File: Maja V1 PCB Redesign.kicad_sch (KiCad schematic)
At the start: 22 parts, among them J1 TYPE-C-31-M-12, J2 AVR-ISP-6, J3 Connector_Generic_Conn_01x04, U1 ATmega32U4-M, U2 PRTR5V0U2X, Y1 Crystal_GND24_Small

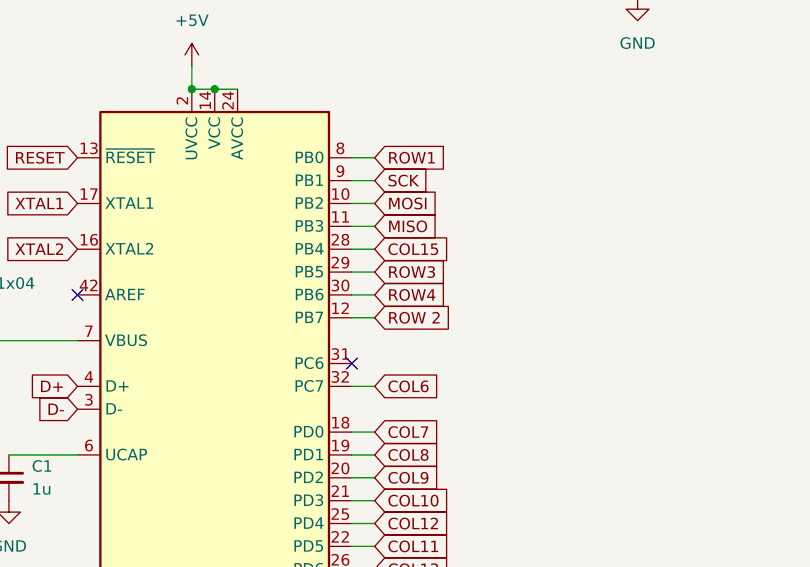
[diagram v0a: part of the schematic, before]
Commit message: routing
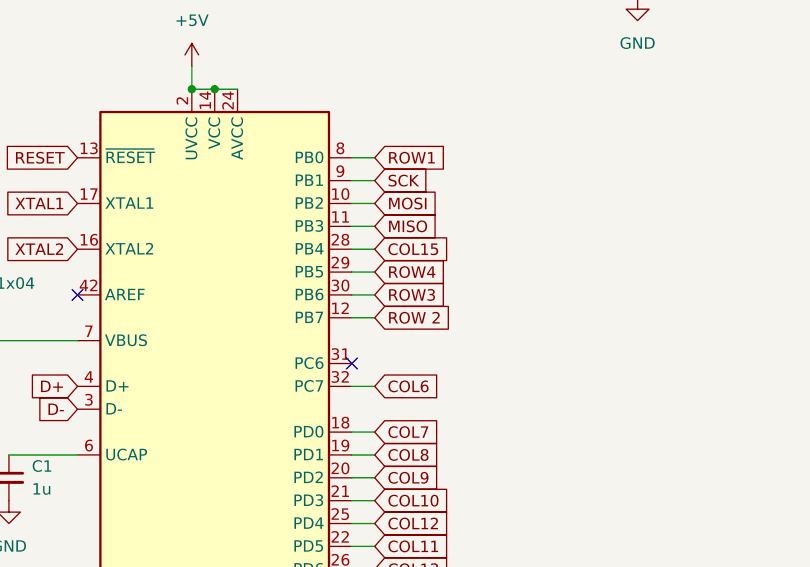
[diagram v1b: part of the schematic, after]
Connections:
- net ROW3: now also U1.30 (PB6); no longer U1.29 (PB5)
- net ROW4: now also U1.29 (PB5); no longer U1.30 (PB6)
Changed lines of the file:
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@@
-    (stroke (width 0) (type default) (color 0 0 0 0))
-  )
-  (wire (pts (xy 177.8 71.12) (xy 175.26 71.12))
     (stroke (width 0) (type default) (color 0 0 0 0))
   )
@@
     (stroke (width 0) (type default) (color 0 0 0 0))
   )
+  (wire (pts (xy 175.26 71.12) (xy 177.8 71.12))
+    (stroke (width 0) (type default) (color 0 0 0 0))
+  )
   (wire (pts (xy 82.55 31.75) (xy 82.55 34.29))
     (stroke (width 0) (type default) (color 0 0 0 0))
@@
     (stroke (width 0) (type default) (color 0 0 0 0))
   )
+  (wire (pts (xy 175.26 73.66) (xy 177.8 73.66))
+    (stroke (width 0) (type default) (color 0 0 0 0))
+  )
   (wire (pts (xy 60.96 116.84) (xy 100.33 116.84))
     (stroke (width 0) (type default) (color 0 0 0 0))
@@
   )
   (wire (pts (xy 241.3 96.52) (xy 241.3 99.06))
-    (stroke (width 0) (type default) (color 0 0 0 0))
-  )
-  (wire (pts (xy 175.26 73.66) (xy 177.8 73.66))
     (stroke (width 0) (type default) (color 0 0 0 0))
   )
@@
     )
   )
-  (global_label "ROW3" (shape input) (at 177.8 71.12 0) (fields_autoplaced)
-    (effects (font (size 1.27 1.27)) (justify left))
-    (property "Intersheet References" "${INTERSHEET_REFS}" (id 0) (at 185.4745 71.1994 0)
+  (global_label "ROW3" (shape input) (at 177.8 73.66 0) (fields_autoplaced)
+    (effects (font (size 1.27 1.27)) (justify left))
+    (property "Intersheet References" "${INTERSHEET_REFS}" (id 0) (at 185.4745 73.7394 0)
       (effects (font (size 1.27 1.27)) (justify left) hide)
     )
@@
     )
   )
-  (global_label "ROW4" (shape input) (at 177.8 73.66 0) (fields_autoplaced)
-    (effects (font (size 1.27 1.27)) (justify left))
-    (property "Intersheet References" "${INTERSHEET_REFS}" (id 0) (at 185.4745 73.7394 0)
-      (effects (font (size 1.27 1.27)) (justify left) hide)
-    )
+  (global_label "ROW4" (shape input) (at 177.8 71.12 0) (fields_autoplaced)
+    (effects (font (size 1.27 1.27)) (justify left))
+    (property "Intersheet References" "${INTERSHEET_REFS}" (id 0) (at 185.4745 71.1994 0)
+      (effects (font (size 1.27 1.27)) (justify left) hide)
+    )

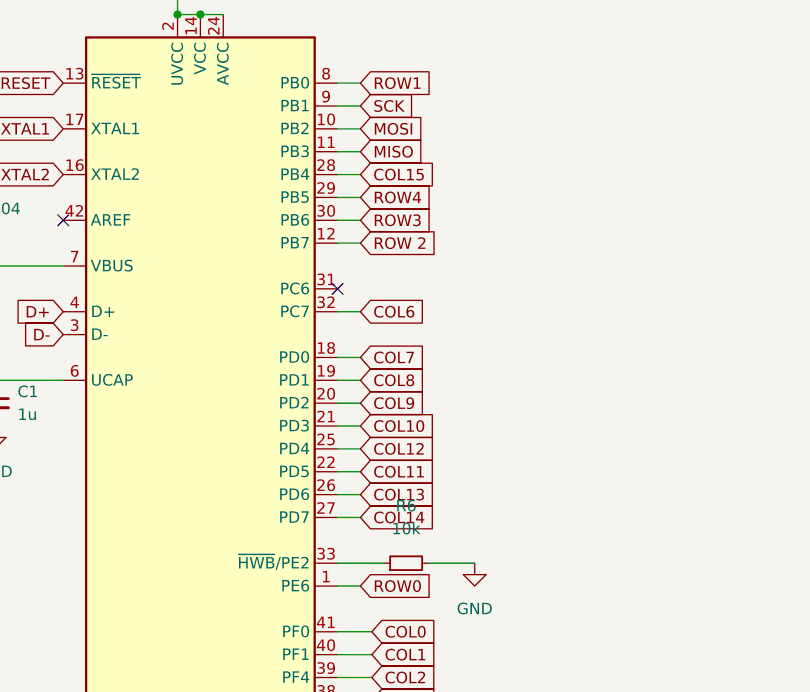
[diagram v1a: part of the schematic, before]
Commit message: routing
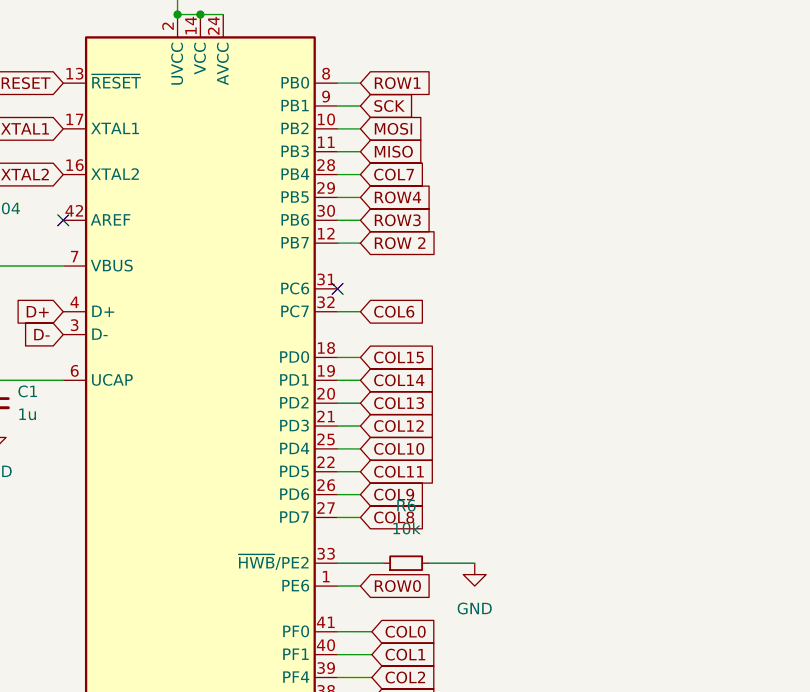
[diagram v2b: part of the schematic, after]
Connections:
- net COL10: now also U1.25 (PD4); no longer U1.21 (PD3)
- net COL12: now also U1.21 (PD3); no longer U1.25 (PD4)
- net COL13: now also U1.20 (PD2); no longer U1.26 (PD6)
- net COL14: now also U1.19 (PD1); no longer U1.27 (PD7)
- net COL15: now also U1.18 (PD0); no longer U1.28 (PB4)
- net COL7: now also U1.28 (PB4); no longer U1.18 (PD0)
- net COL8: now also U1.27 (PD7); no longer U1.19 (PD1)
- net COL9: now also U1.26 (PD6); no longer U1.20 (PD2)

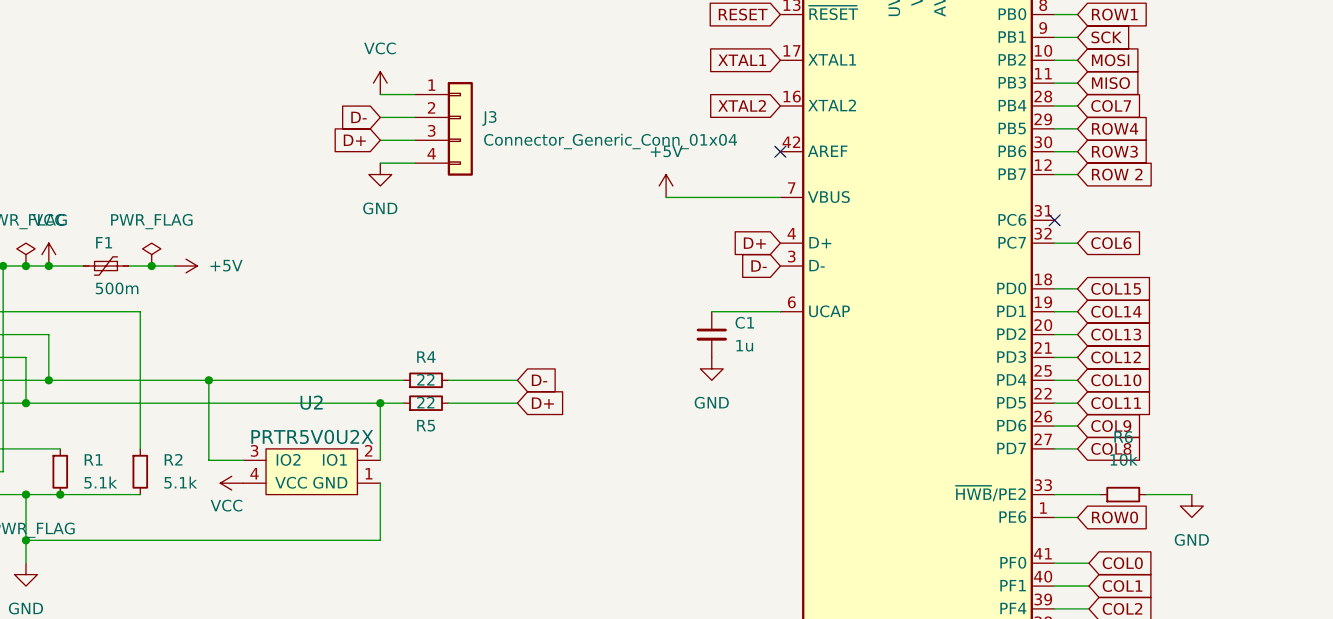
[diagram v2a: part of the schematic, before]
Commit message: routing
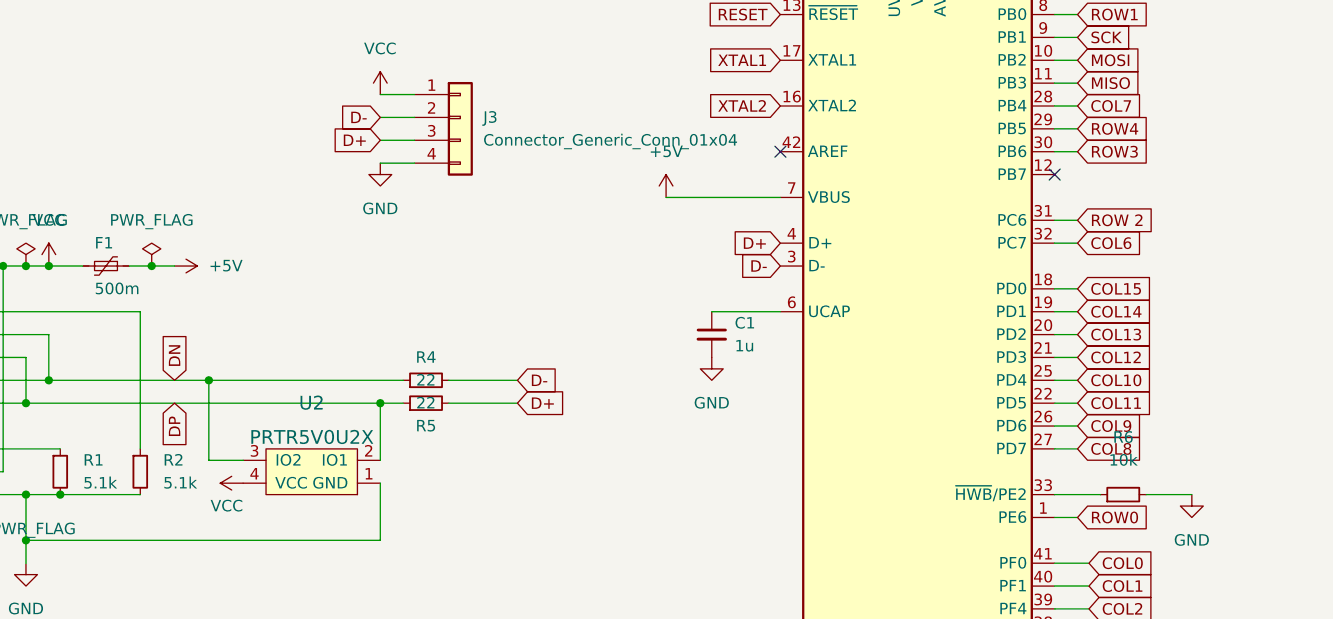
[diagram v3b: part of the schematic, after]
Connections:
- net ROW 2: now also U1.31 (PC6); no longer U1.12 (PB7)
- net DP: now reaches J1.A6 (DP1), J1.B6 (DP2), R5.1, U2.2 (IO1)
- net DN: now reaches J1.A7 (DN1), J1.B7 (DN2), R4.1, U2.3 (IO2)
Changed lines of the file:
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@@
   (no_connect (at 78.74 39.37))
   (no_connect (at 144.78 73.66))
-  (no_connect (at 175.26 81.28))
   (no_connect (at 53.34 104.14))
   (no_connect (at 53.34 88.9))
+  (no_connect (at 175.26 76.2))
   (no_connect (at 63.5 34.29))
   (wire (pts (xy 175.26 91.44) (xy 177.8 91.44))
@@
     (stroke (width 0) (type default) (color 0 0 0 0))
   )
-  (wire (pts (xy 175.26 76.2) (xy 177.8 76.2))
-    (stroke (width 0) (type default) (color 0 0 0 0))
-  )
   (wire (pts (xy 53.34 96.52) (xy 60.96 96.52))
     (stroke (width 0) (type default) (color 0 0 0 0))
@@
   )
   (wire (pts (xy 147.32 142.24) (xy 157.48 142.24))
+    (stroke (width 0) (type default) (color 0 0 0 0))
+  )
+  (wire (pts (xy 175.26 81.28) (xy 177.8 81.28))
     (stroke (width 0) (type default) (color 0 0 0 0))
   )
@@
     )
   )
-  (global_label "ROW 2" (shape input) (at 177.8 76.2 0) (fields_autoplaced)
-    (effects (font (size 1.27 1.27)) (justify left))
-    (property "Intersheet References" "${INTERSHEET_REFS}" (id 0) (at 186.4421 76.2794 0)
+  (global_label "ROW 2" (shape input) (at 177.8 81.28 0) (fields_autoplaced)
+    (effects (font (size 1.27 1.27)) (justify left))
+    (property "Intersheet References" "${INTERSHEET_REFS}" (id 0) (at 186.4421 81.3594 0)
       (effects (font (size 1.27 1.27)) (justify left) hide)
     )
@@
     )
   )
+  (global_label "DP" (shape input) (at 77.47 101.6 270) (fields_autoplaced)
+    (effects (font (size 1.27 1.27)) (justify right))
+    (property "Intersheet References" "${INTERSHEET_REFS}" (id 0) (at 77.3906 106.5531 90)
+      (effects (font (size 1.27 1.27)) (justify right) hide)
+    )
+  )
   (global_label "RESET" (shape input) (at 144.78 58.42 180) (fields_autoplaced)
     (effects (font (size 1.27 1.27)) (justify right))
@@
       (effects (font (size 1.27 1.27)) (justify left) hide)
     )
+  )
+  (global_label "DN" (shape input) (at 77.47 99.06 90) (fields_autoplaced)
+    (effects (font (size 1.27 1.27)) (justify left))
+    (property "Intersheet References" "${INTERSHEET_REFS}" (id 0) (at 77.3906 94.0464 90)
+      (effects (font (size 1.27 1.27)) (justify left) hide)
+    )

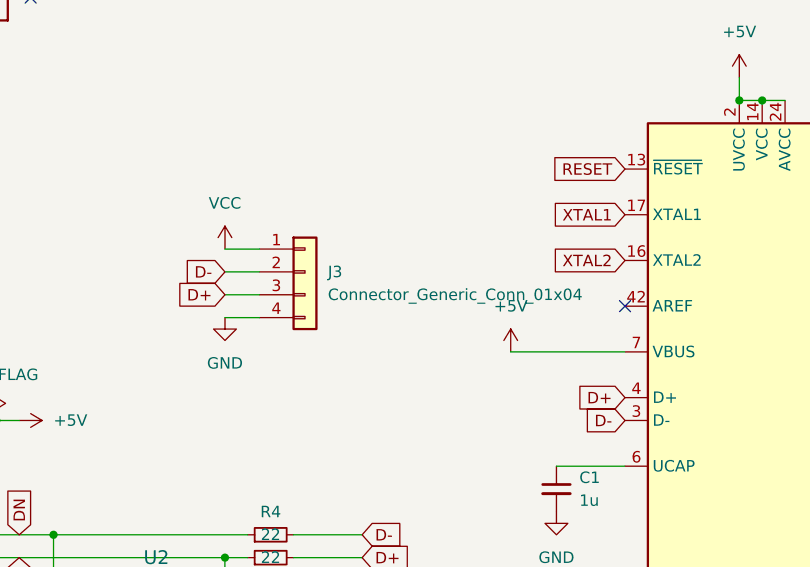
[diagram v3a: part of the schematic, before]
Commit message: ROUTING DONE
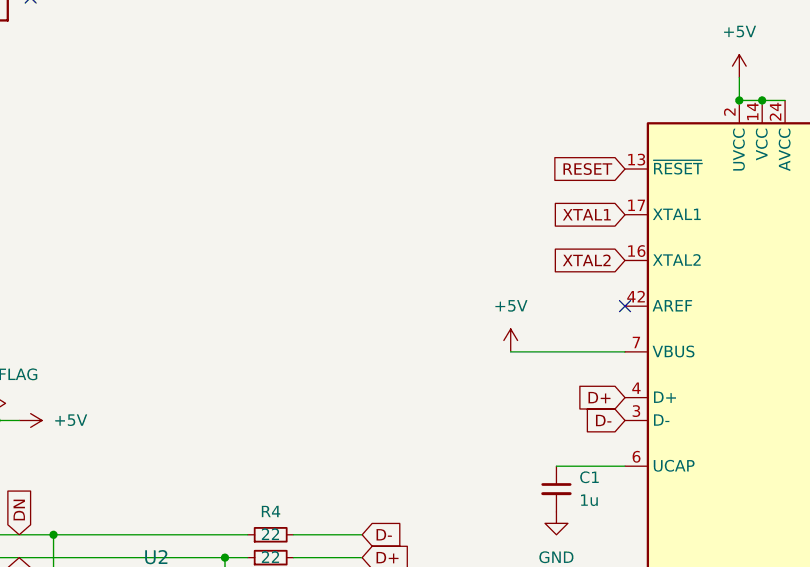
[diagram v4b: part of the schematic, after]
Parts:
- removed J3: Connector_Generic_Conn_01x04, Connector_JST:JST_SH_SM04B-SRSS-TB_1x04-1MP_P1.00mm_Horizontal, symbol Unified-Daughterboard-cache:Connector_Generic_Conn_01x04
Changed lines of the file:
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@@
-    (stroke (width 0) (type default) (color 0 0 0 0))
-  )
-  (wire (pts (xy 100.33 69.85) (xy 104.14 69.85))
-    (stroke (width 0) (type default) (color 0 0 0 0))
-  )
-  (wire (pts (xy 100.33 72.39) (xy 104.14 72.39))
     (stroke (width 0) (type default) (color 0 0 0 0))
   )
@@
     (stroke (width 0) (type default) (color 0 0 0 0))
   )
-  (wire (pts (xy 100.33 74.93) (xy 104.14 74.93))
-    (stroke (width 0) (type default) (color 0 0 0 0))
-  )
   (wire (pts (xy 160.02 50.8) (xy 162.56 50.8))
     (stroke (width 0) (type default) (color 0 0 0 0))
@@
   )
   (wire (pts (xy 234.95 82.55) (xy 234.95 88.9))
-    (stroke (width 0) (type default) (color 0 0 0 0))
-  )
-  (wire (pts (xy 100.33 67.31) (xy 104.14 67.31))
     (stroke (width 0) (type default) (color 0 0 0 0))
   )
@@
     )
   )
-  (global_label "D-" (shape input) (at 100.33 69.85 180) (fields_autoplaced)
-    (effects (font (size 1.27 1.27)) (justify right))
-    (property "Intersheet References" "${INTERSHEET_REFS}" (id 0) (at 95.0745 69.7706 0)
-      (effects (font (size 1.27 1.27)) (justify right) hide)
-    )
-  )
   (global_label "SCK" (shape input) (at 219.71 30.48 0) (fields_autoplaced)
     (effects (font (size 1.27 1.27)) (justify left))
@@
     (property "Intersheet References" "${INTERSHEET_REFS}" (id 0) (at 183.9626 60.8806 0)
       (effects (font (size 1.27 1.27)) (justify left) hide)
-    )
-  )
-  (global_label "D+" (shape input) (at 100.33 72.39 180) (fields_autoplaced)
-    (effects (font (size 1.27 1.27)) (justify right))
-    (property "Intersheet References" "${INTERSHEET_REFS}" (id 0) (at 95.0745 72.3106 0)
-      (effects (font (size 1.27 1.27)) (justify right) hide)
     )
   )
@@
     (pin "S4")
   )
-  (symbol (lib_id "Unified-Daughterboard-cache:Connector_Generic_Conn_01x04") (at 109.22 69.85 0) (unit 1)
-    (in_bom yes) (on_board yes) (fields_autoplaced)
-    (property "Reference" "J3" (id 0) (at 111.76 69.8499 0)
-      (effects (font (size 1.27 1.27)) (justify left))
-    )
-    (property "Value" "Connector_Generic_Conn_01x04" (id 1) (at 111.76 72.3899 0)
-      (effects (font (size 1.27 1.27)) (justify left))
-    )
-    (property "Footprint" "Connector_JST:JST_SH_SM04B-SRSS-TB_1x04-1MP_P1.00mm_Horizontal" (id 2) (at 109.22 69.85 0)
-      (effects (font (size 1.27 1.27)) hide)
-    )
-    (property "Datasheet" "" (id 3) (at 109.22 69.85 0)
-      (effects (font (size 1.27 1.27)) hide)
-    )
-    (pin "1")
-    (pin "2")
-    (pin "3")
-    (pin "4")
-  )
   (symbol (lib_id "power:GND") (at 190.5 111.76 0) (unit 1)
     (in_bom yes) (on_board yes) (fields_autoplaced)
@@
     (pin "1")
     (pin "2")
-  )
-  (symbol (lib_id "power:VCC") (at 100.33 67.31 0) (unit 1)
-    (in_bom yes) (on_board yes) (fields_autoplaced)
-    (property "Reference" "#PWR0117" (id 0) (at 100.33 71.12 0)
-      (effects (font (size 1.27 1.27)) hide)
-    )
-    (property "Value" "VCC" (id 1) (at 100.33 62.23 0))
-    (property "Footprint" "" (id 2) (at 100.33 67.31 0)
-      (effects (font (size 1.27 1.27)) hide)
-    )
-    (property "Datasheet" "" (id 3) (at 100.33 67.31 0)
-      (effects (font (size 1.27 1.27)) hide)
-    )
-    (pin "1")
-  )
-  (symbol (lib_id "power:GND") (at 100.33 74.93 0) (unit 1)
-    (in_bom yes) (on_board yes) (fields_autoplaced)
-    (property "Reference" "#PWR0118" (id 0) (at 100.33 81.28 0)
-      (effects (font (size 1.27 1.27)) hide)
-    )
-    (property "Value" "GND" (id 1) (at 100.33 80.01 0))
-    (property "Footprint" "" (id 2) (at 100.33 74.93 0)
-      (effects (font (size 1.27 1.27)) hide)
-    )
-    (property "Datasheet" "" (id 3) (at 100.33 74.93 0)
-      (effects (font (size 1.27 1.27)) hide)
-    )
-    (pin "1")
   )
   (symbol (lib_id "power:+5V") (at 132.08 78.74 0) (unit 1)
@@
       (reference "#PWR0116") (unit 1) (value "+5V") (footprint "")
     )
-    (path "/468ba756-b608-4ef3-b75b-cee3864ffcfd"
-      (reference "#PWR0117") (unit 1) (value "VCC") (footprint "")
-    )
-    (path "/47139887-f780-4c14-afae-8d820d1e0de6"
-      (reference "#PWR0118") (unit 1) (value "GND") (footprint "")
-    )
     (path "/43d87709-5a30-4180-96d5-6f8b8ffdfd1d"
       (reference "C1") (unit 1) (value "1u") (footprint "Capacitor_SMD:C_0805_2012Metric_Pad1.18x1.45mm_HandSolder")
@@
       (reference "J2") (unit 1) (value "AVR-ISP-6") (footprint "random-keyboard-parts:Reset_Pretty")
     )
-    (path "/361725fc-4f2d-472a-8075-f63ed1495c22"
-      (reference "J3") (unit 1) (value "Connector_Generic_Conn_01x04") (footprint "Connector_JST:JST_SH_SM04B-SRSS-TB_1x04-1MP_P1.00mm_Horizontal")
-    )
     (path "/4526e43e-053f-4520-ab68-78d672909c1b/574f6d28-bfb7-4f6c-b7f3-59d6bbd5a2c5"
